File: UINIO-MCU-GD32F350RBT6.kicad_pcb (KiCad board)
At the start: 2 copper layers, 0 parts

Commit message: Finish PCB layout.
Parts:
- added C1: 1uF, Capacitor_SMD:C_0603_1608Metric, F.Cu at (157.9, 130.8)
- added C10: 20pF, Capacitor_SMD:C_0603_1608Metric, F.Cu at (145.9, 124.0)
- added C2: 0.1uF, Capacitor_SMD:C_0603_1608Metric, F.Cu at (104.4, 130.7)
- added C3: 1uF, Capacitor_SMD:C_0603_1608Metric, F.Cu at (151.7, 130.8)
- added C4: 0.1uF, Capacitor_SMD:C_0603_1608Metric, F.Cu at (137.7, 129.6)
- added C5: 0.1uF, Capacitor_SMD:C_0603_1608Metric, F.Cu at (118.2, 130.8)
- added C6: 20pF, Capacitor_SMD:C_0603_1608Metric, F.Cu at (145.9, 126.0)
- added C7: 0.1uF, Capacitor_SMD:C_0603_1608Metric, F.Cu at (104.4, 124.8)
- added C8: 10pF, Capacitor_SMD:C_0603_1608Metric, F.Cu at (144.8, 131.7)
- added C9: 10pF, Capacitor_SMD:C_0603_1608Metric, F.Cu at (144.8, 129.2)
- added D1: LED_Red, LED_SMD:LED_0603_1608Metric, F.Cu at (153.1, 123.9)
- added HOLE**: Hole-1mm, Uinio:Hole-1mm, F.Cu at (161.0, 132.2)
- added HOLE**: Hole-1mm, Uinio:Hole-1mm, F.Cu at (97.3, 124.1)
- added HOLE**: Hole-1mm, Uinio:Hole-1mm, F.Cu at (97.3, 131.7)
- added HOLE**: Hole-1mm, Uinio:Hole-1mm, F.Cu at (161.0, 123.6)
- added J1: Conn_01x32_Male, Connector_PinHeader_2.54mm:PinHeader_1x32_P2.54mm_Vertical, B.Cu at (169.7, 118.9)
- added J2: Conn_01x32_Male, Connector_PinHeader_2.54mm:PinHeader_1x32_P2.54mm_Vertical, B.Cu at (169.7, 136.8)
- added J3: Conn_01x04_Male, Connector_PinHeader_2.54mm:PinHeader_1x04_P2.54mm_Vertical, F.Cu at (91.0, 131.7)
- added L1: 1KΩ 100Mhz, Inductor_SMD:L_0603_1608Metric, F.Cu at (118.2, 124.8)
- added R1: 2K, Resistor_SMD:R_0603_1608Metric, F.Cu at (156.1, 123.9)
- added R2: 10K, Resistor_SMD:R_0603_1608Metric, F.Cu at (116.2, 130.8)
- added R3: 10K, Resistor_SMD:R_0603_1608Metric, F.Cu at (116.2, 124.8)
- added R4: 1M, Resistor_SMD:R_0603_1608Metric, F.Cu at (139.2, 125.0)
- added R5: 10K, Resistor_SMD:R_0603_1608Metric, F.Cu at (102.5, 130.7)
- added R6: 10K, Resistor_SMD:R_0603_1608Metric, F.Cu at (102.5, 124.8)
- added R7: 50R, Resistor_SMD:R_0603_1608Metric, F.Cu at (156.1, 126.8)
- added R8: 50R, Resistor_SMD:R_0603_1608Metric, F.Cu at (156.1, 125.4)
- added R9: 1.5K, Resistor_SMD:R_0603_1608Metric, F.Cu at (156.1, 128.3)
- added SW1: BOOT0, Uinio:KEY-SMD_4P-L4.2-W3.4-P2.15-LS4.7, F.Cu at (109.7, 130.8)
- added SW2: NRST, Uinio:KEY-SMD_4P-L4.2-W3.4-P2.15-LS4.7, F.Cu at (109.7, 124.8)
- added U1: ME6211C33M5G-N, Uinio:SOT-23-5_L3.0-W1.7-P0.95-LS2.8-BR, F.Cu at (154.8, 130.9)
- added U2: GD32F350RBT6, Uinio:LQFP-64_L10.0-W10.0-P0.50-LS12.0-BL, F.Cu at (127.8, 127.9)
- added USB1: USB_Type_C_16Pin, Uinio:USB-C-SMD_TYPEC-304J-BCP16, F.Cu at (166.5, 127.9)
- added Y1: 32.768KHz, Uinio:CRYSTAL-FC135-32.768, F.Cu at (142.2, 130.5)
- added Y2: 8MHz, Crystal:Crystal_SMD_3225-4Pin_3.2x2.5mm, F.Cu at (142.2, 125.0)
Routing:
- net /VSSA: track 0.00 -> 16.0 mm
- net /PA12: track 0.00 -> 1.46 mm
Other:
- board outline added: 81.5 x 20.5 mm
- board text added: "3.3V"
- board text added: "A10"
- board text added: "A11"
- board text added: "A12"
- board text added: "A13"
- board text added: "A13/SWDIO"
- board text added: "A14"
- board text added: "A14/SWCLK"
- board text added: "A15"
- board text added: "A3"
- board text added: "BOOT0"
- board text added: "F4"
- board text added: "F6"
- board text added: "F7"
- board text added: "GND"
- board text added: "NRST"

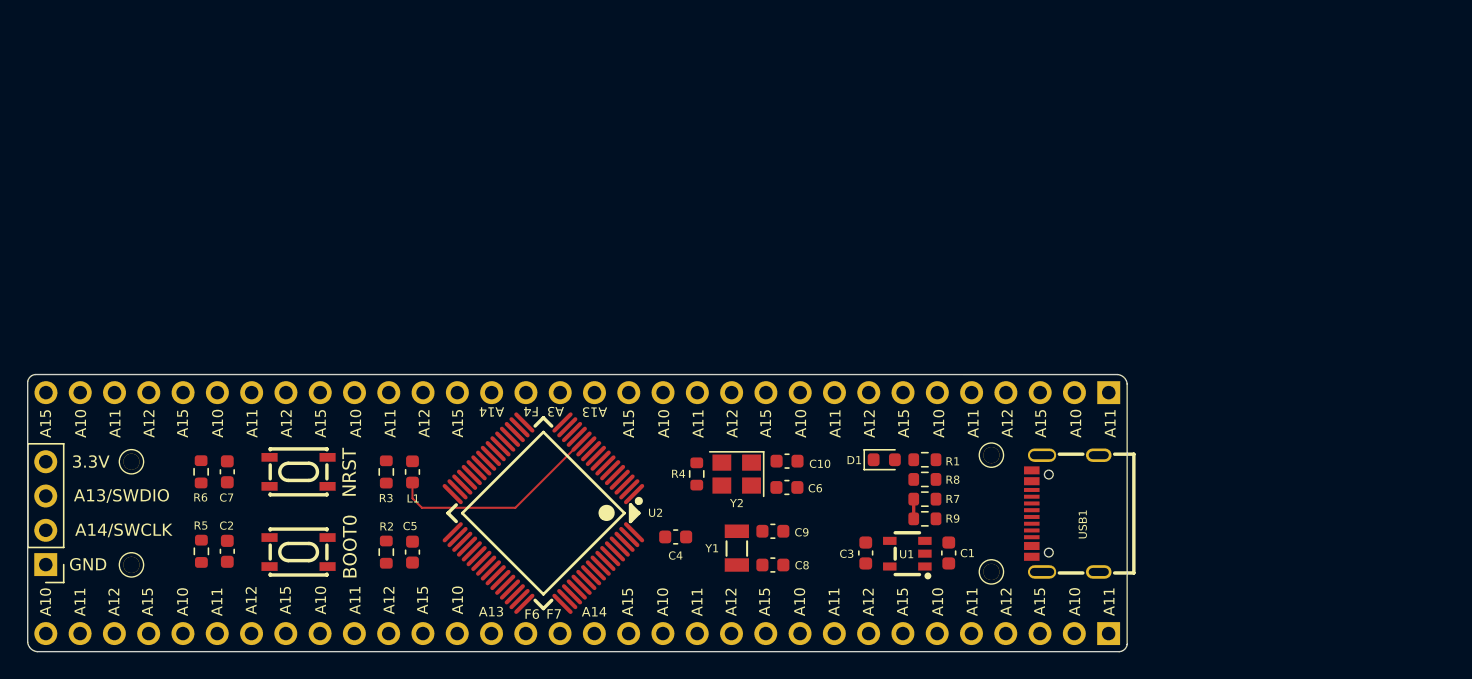
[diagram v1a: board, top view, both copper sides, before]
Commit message: Finish PCB layout.
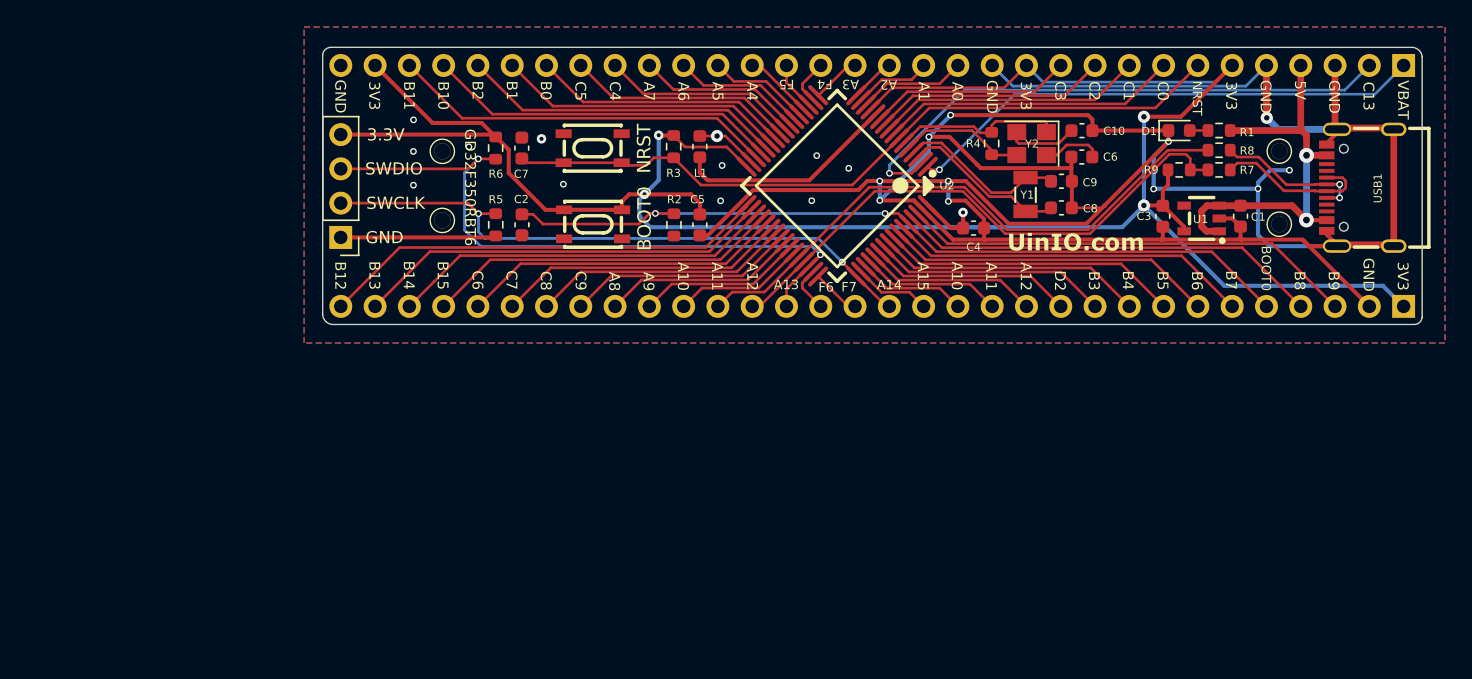
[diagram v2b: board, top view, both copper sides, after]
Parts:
- removed HOLE** (x3): Hole-1mm, Uinio:Hole-1mm
- added ?: LOGO, LOGO, F.Cu at (167.3, 107.8)
- added ?: LOGO, LOGO, B.Cu at (169.7, 103.8)
- added ?: LOGO, LOGO, B.Cu at (142.8, 103.5)
- added HOLE1: Hole-1mm, Uinio:Hole-1mm, F.Cu at (120.4, 101.1)
- added HOLE2: Hole-1mm, Uinio:Hole-1mm, F.Cu at (120.4, 106.2)
- added HOLE3: Hole-1mm, Uinio:Hole-1mm, F.Cu at (182.4, 101.0)
- moved C8 34.0 mm to (166.2, 105.2), turned to 180 degrees
- moved Y1 33.8 mm to (163.6, 104.3)
- moved C9 33.6 mm to (166.2, 103.3)
- moved C3 33.3 mm to (173.7, 105.9), turned to 90 degrees
- moved U1 33.0 mm to (176.6, 106.0)
- moved C1 33.0 mm to (179.5, 105.9)
- moved C6 32.8 mm to (167.7, 101.5)
- moved Y2 32.8 mm to (164.0, 100.5)
- moved C10 32.8 mm to (167.8, 99.5), turned to 180 degrees
- moved R4 32.8 mm to (161.1, 100.5)
- moved D1 32.7 mm to (174.9, 99.5)
- moved R1 32.7 mm to (177.9, 99.5)
- moved R7 32.7 mm to (177.9, 102.4)
- moved R8 32.7 mm to (177.9, 101.0)
- moved SW1 32.6 mm to (131.5, 106.5)
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- renumbered HOLE** to HOLE4
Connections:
- J1 pad 31: /VDD_5V -> /VDD_3.3V
- J1 pad 4: /VDD_3.3V -> /VDD_5V
- J1 pad 5: /VDD_3.3V -> GND
- J1 pad 6: GND -> /VDD_3.3V
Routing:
- net GND: track 0.00 -> 233.5 mm, vias 0 -> 23
- net /VDD_3.3V: track 0.00 -> 179.1 mm, vias 0 -> 5
- net /BOOT0: track 0.00 -> 60.0 mm, vias 0 -> 2
- net /NRST: track 0.00 -> 54.5 mm
- net /PA13/SWDIO: track 0.00 -> 49.4 mm, vias 0 -> 2
- net /PA14/SWCLK: track 0.00 -> 45.6 mm, vias 0 -> 2
- net /PA11: track 0.00 -> 43.7 mm
- net /PC13: track 0.00 -> 42.0 mm, vias 0 -> 1
- net /PA12: track 1.46 -> 41.5 mm
- net /VBAT: track 0.00 -> 38.5 mm, vias 0 -> 1
- net /PB9: track 0.00 -> 33.7 mm
- net /PB12: track 0.00 -> 33.2 mm
- net /PB8: track 0.00 -> 31.4 mm
- net /VDD_5V: track 0.00 -> 30.9 mm, vias 0 -> 2
- net /PB13: track 0.00 -> 30.8 mm
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- added copper zone on B.Cu, net GND
- added copper zone on F.Cu, net GND
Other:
- board text added: "3V3"
- board text added: "5V"
- board text added: "A0"
- board text added: "A1"
- board text added: "A2"
- board text added: "A4"
- board text added: "A5"
- board text added: "A6"
- board text added: "A7"
- board text added: "A8"
- board text added: "A9"
- board text added: "B0"
- board text added: "B1"
- board text added: "B10"
- board text added: "B11"
- board text added: "B12"
- board text added: "B13"
- board text added: "B14"
- board text added: "B15"
- board text added: "B2"
- board text added: "B3"
- board text added: "B4"
- board text added: "B5"
- board text added: "B6"
- board text added: "B7"
- board text added: "B8"
- board text added: "B9"
- board text added: "C0"
- board text added: "C1"
- board text added: "C13"
- board text added: "C2"
- board text added: "C3"
- board text added: "C4"
- board text added: "C5"
- board text added: "C6"
- board text added: "C7"
- board text added: "C8"
- board text added: "C9"
- board text added: "D2"
- board text added: "F5"
- board text added: "GD32F350RBT6"
- board text added: "SWCLK"
- board text added: "SWDIO"
- board text added: "UINIO-MCU-GD32F350RBT6"
- board text added: "VBAT"
- board text added: "Version 1.0.0"
- board text removed: "A13/SWDIO"
- board text removed: "A14/SWCLK"
